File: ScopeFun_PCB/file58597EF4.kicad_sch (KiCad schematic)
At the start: 27 parts, among them U36 IS43TR16256B-125KBL

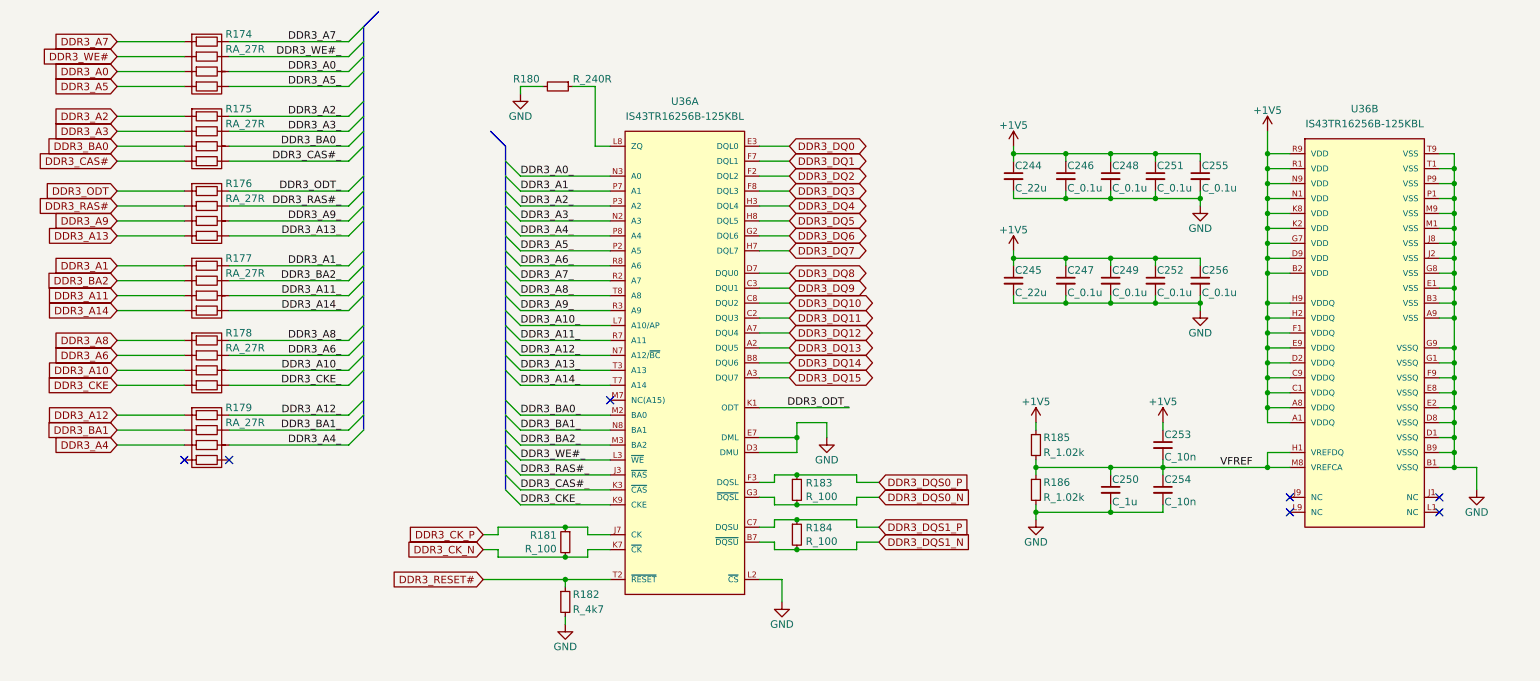
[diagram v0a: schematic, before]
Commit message: 260420
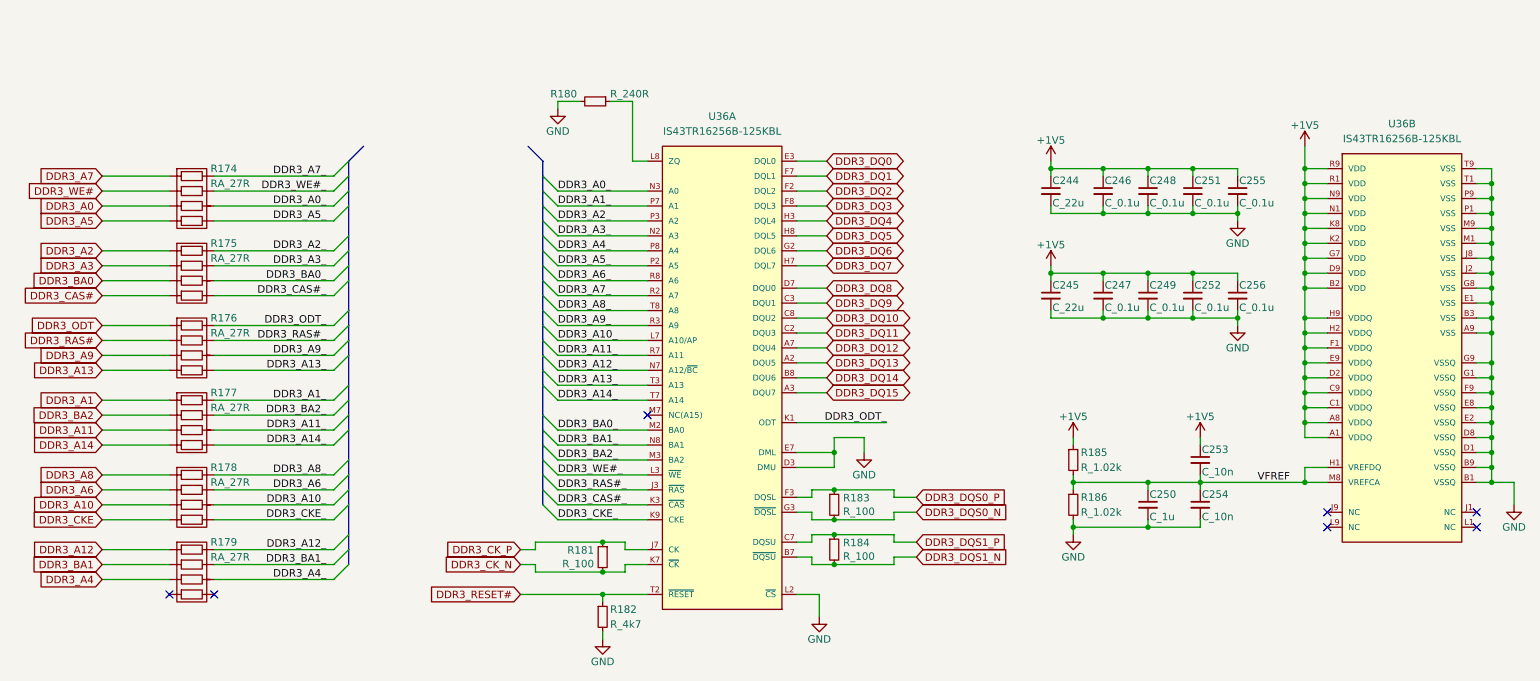
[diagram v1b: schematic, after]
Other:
- moved on the sheet: C244, C245, C246, C247, C248, C249, C250, C251, C252, C253, C254, C255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
